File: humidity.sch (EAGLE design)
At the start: 9 parts

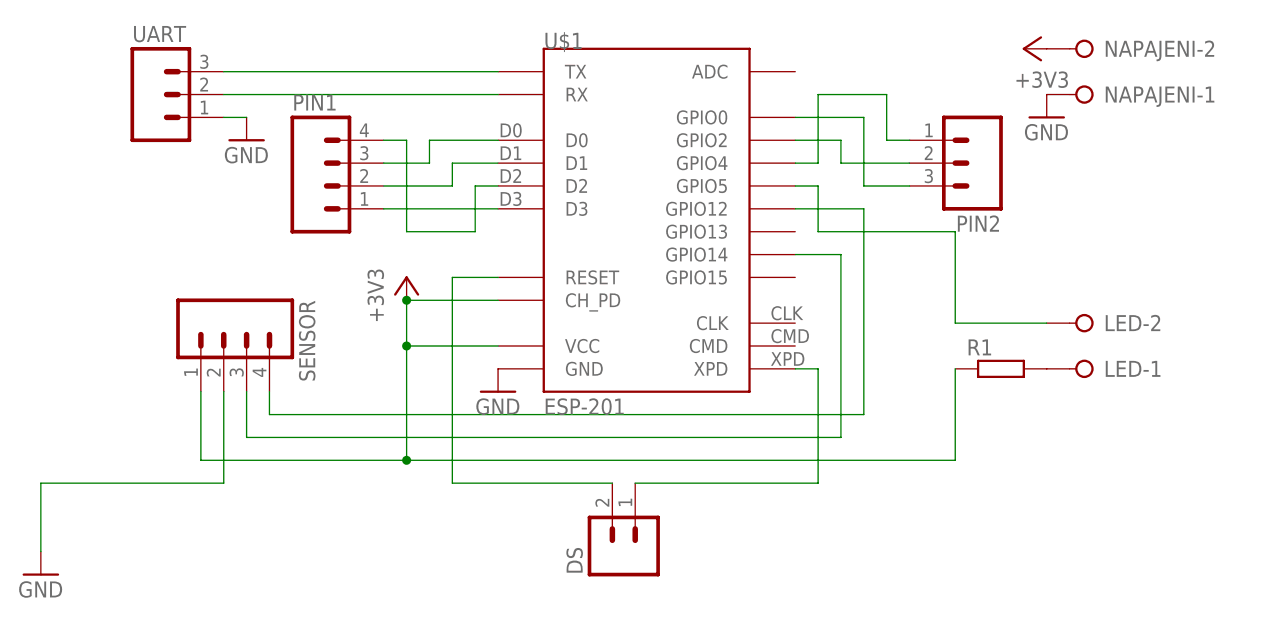
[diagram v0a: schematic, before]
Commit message: DPS
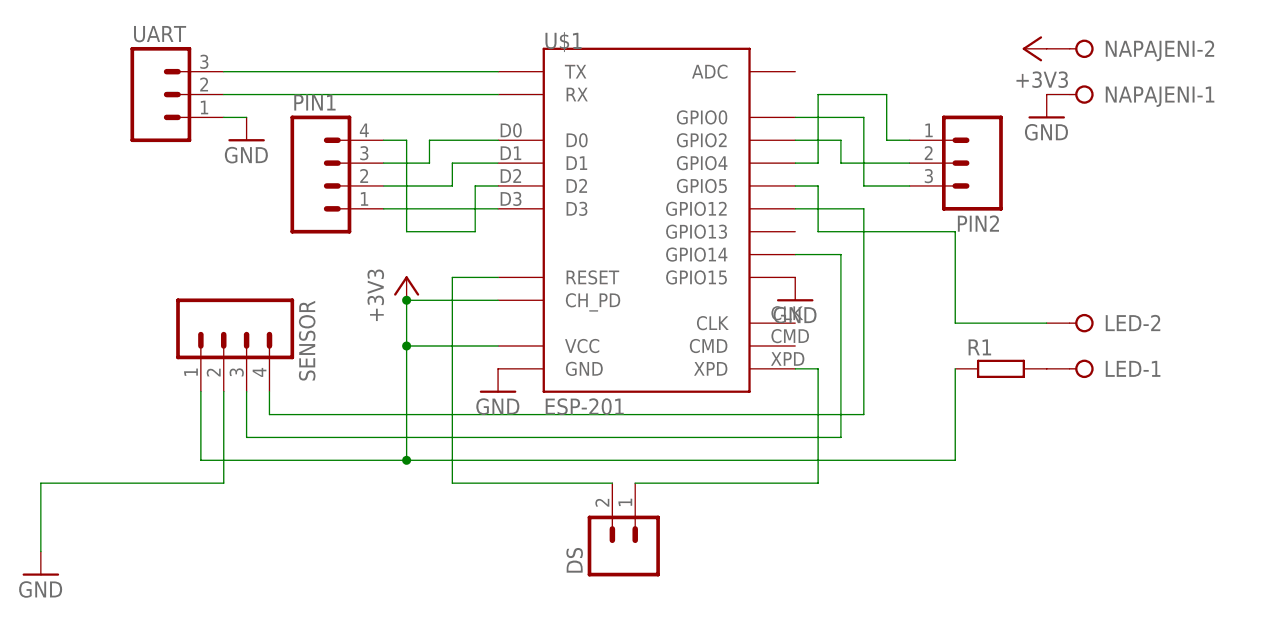
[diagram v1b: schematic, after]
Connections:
- net GND: now also U$1.GPIO15
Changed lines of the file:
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@@
 <?xml version="1.0" encoding="utf-8"?>
 <!DOCTYPE eagle SYSTEM "eagle.dtd">
-<eagle version="6.5.0">
+<eagle version="7.3.0">
 <drawing>
 <settings>
@@
 <part name="R1" library="rcl" deviceset="R-EU_" device="0207/7"/>
 <part name="LED" library="con-wago-508" deviceset="W237-02P" device=""/>
+<part name="GND5" library="supply1" deviceset="GND" device=""/>
 </parts>
 <sheets>
@@
 <instance part="LED" gate="-1" x="144.78" y="88.9" rot="R180"/>
 <instance part="LED" gate="-2" x="144.78" y="93.98" rot="R180"/>
+<instance part="GND5" gate="1" x="111.76" y="96.52"/>
 </instances>
 <busses>
@@
 <pinref part="GND4" gate="1" pin="GND"/>
 </segment>
+<segment>
+<pinref part="U$1" gate="G$1" pin="GPIO15"/>
+<pinref part="GND5" gate="1" pin="GND"/>
+</segment>
 </net>
